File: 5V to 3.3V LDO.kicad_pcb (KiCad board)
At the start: 2 copper layers, 20.4 x 17.8 mm, 9 parts, among them J1 Conn_01x02_Pin, J2 Conn_01x02_Pin, U1 AMS1117-3.3

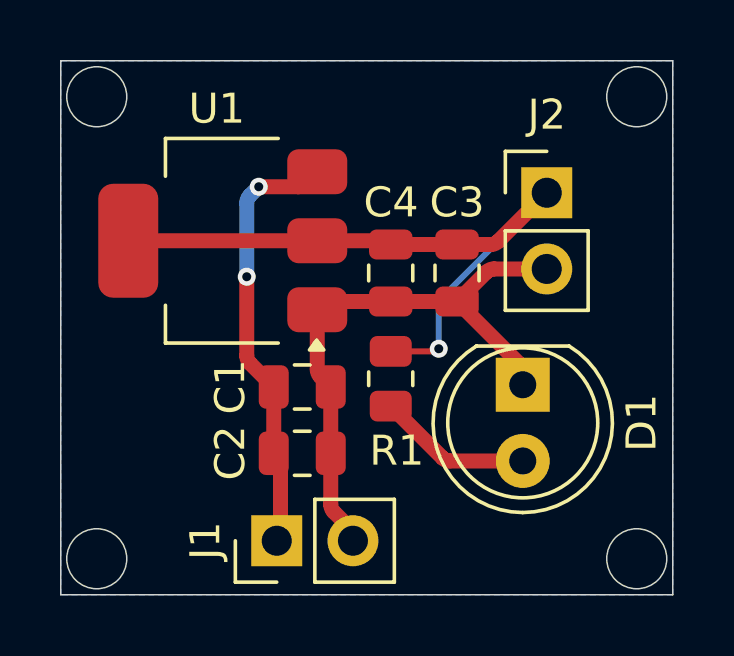
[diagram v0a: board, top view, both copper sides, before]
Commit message: Updated KiCad project and PCB files
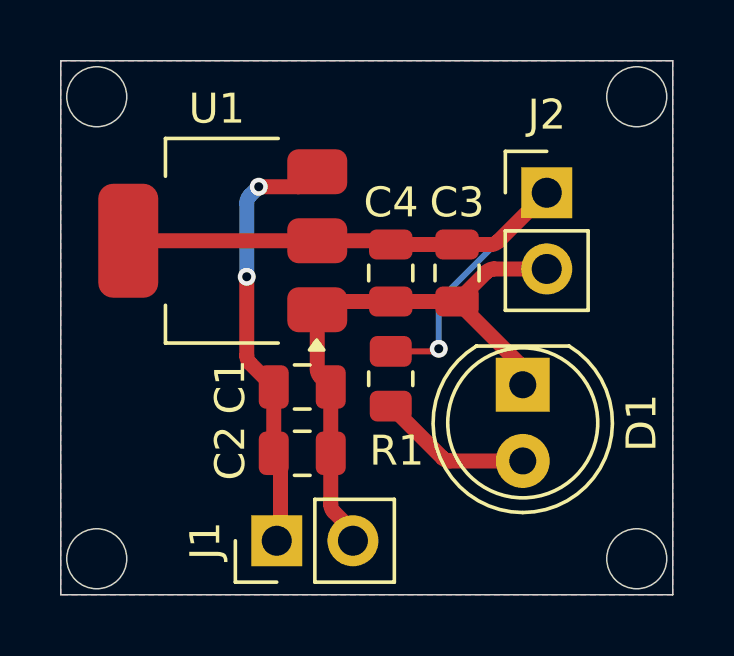
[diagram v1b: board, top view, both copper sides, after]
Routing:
- added copper zone on F.Cu, net GND
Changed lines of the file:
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@@
 	(zone
 		(net "GND")
-		(layer "B.Cu")
+		(layers "F.Cu" "B.Cu")
 		(hatch edge 0.5)
 		(connect_pads
